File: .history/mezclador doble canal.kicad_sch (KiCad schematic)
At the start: 40 parts, among them J1 Conn_Coaxial, J3 Conn_Coaxial, J4 Conn_Coaxial, J5 Conn_Coaxial, J7 Screw_Terminal_01x02, J8 Conn_Coaxial, SW1 SW_SPST, U1 NE5532, U2 TL071

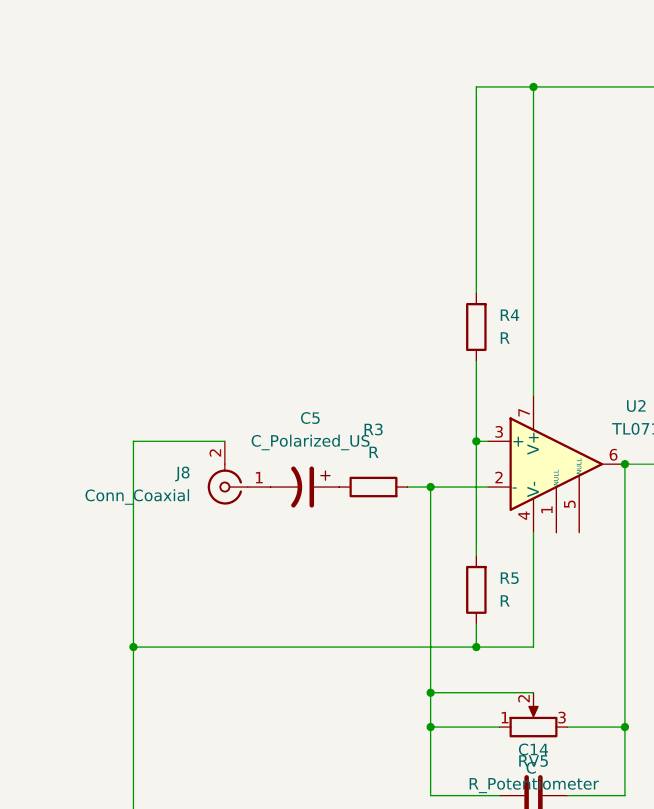
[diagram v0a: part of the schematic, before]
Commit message: acomodando componentes
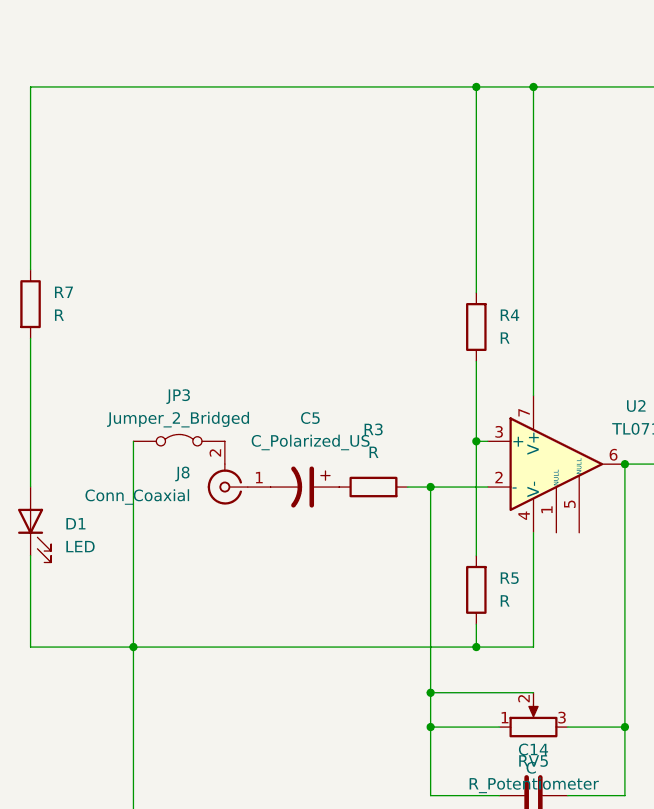
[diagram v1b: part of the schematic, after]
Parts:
- added D1: LED, LED_THT:LED_D5.0mm, symbol Device:LED
- added JP3: Jumper_2_Bridged, personal:Jumper_Wire_7mm, symbol Jumper:Jumper_2_Bridged
- added R7: R, Resistor_THT:R_Axial_DIN0207_L6.3mm_D2.5mm_P7.62mm_Horizontal, symbol Device:R
- JP2: footprint personal:Jumper_Wire_10mm -> personal:Jumper_Wire_7mm
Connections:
- net GND: now also D1.1 (K), JP3.1 (A); no longer J8.2 (Ext)
- net VCC: now also R7.1
- new net: J8.2 (Ext), JP3.2 (B)
- new net: D1.2 (A), R7.2

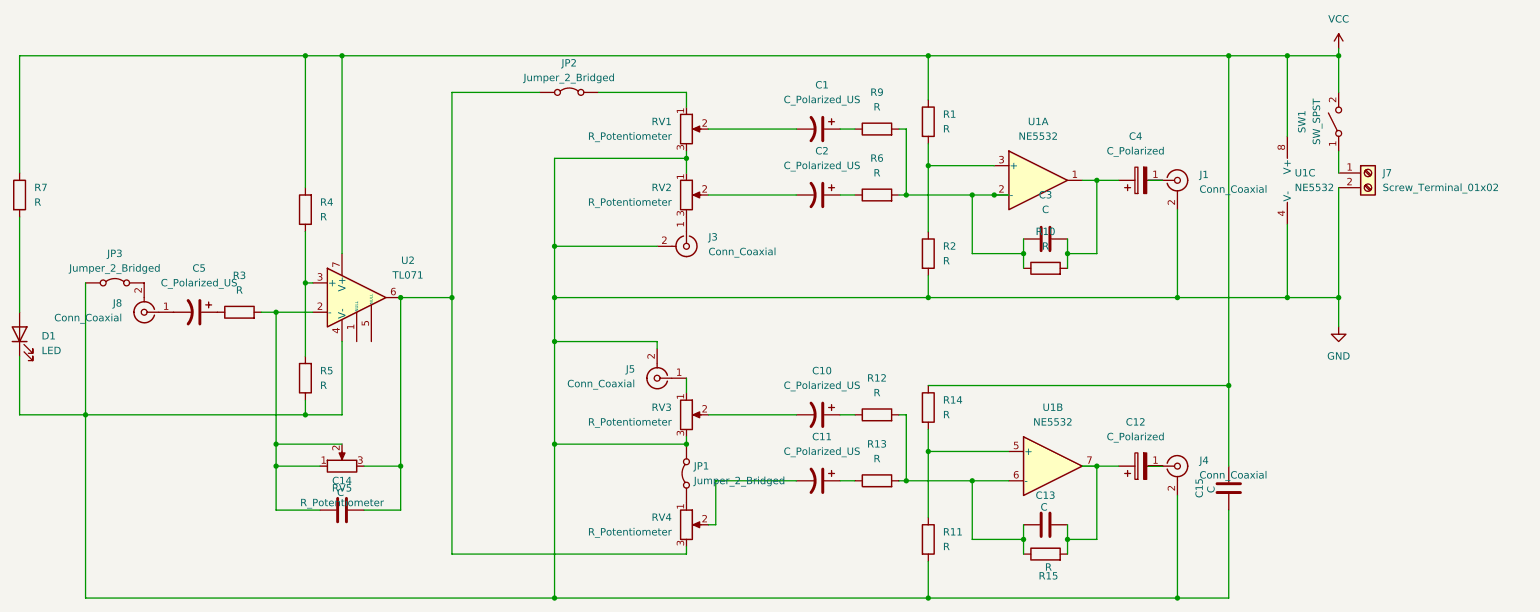
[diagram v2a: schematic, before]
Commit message: todo en su lugar / tamaño 50x55
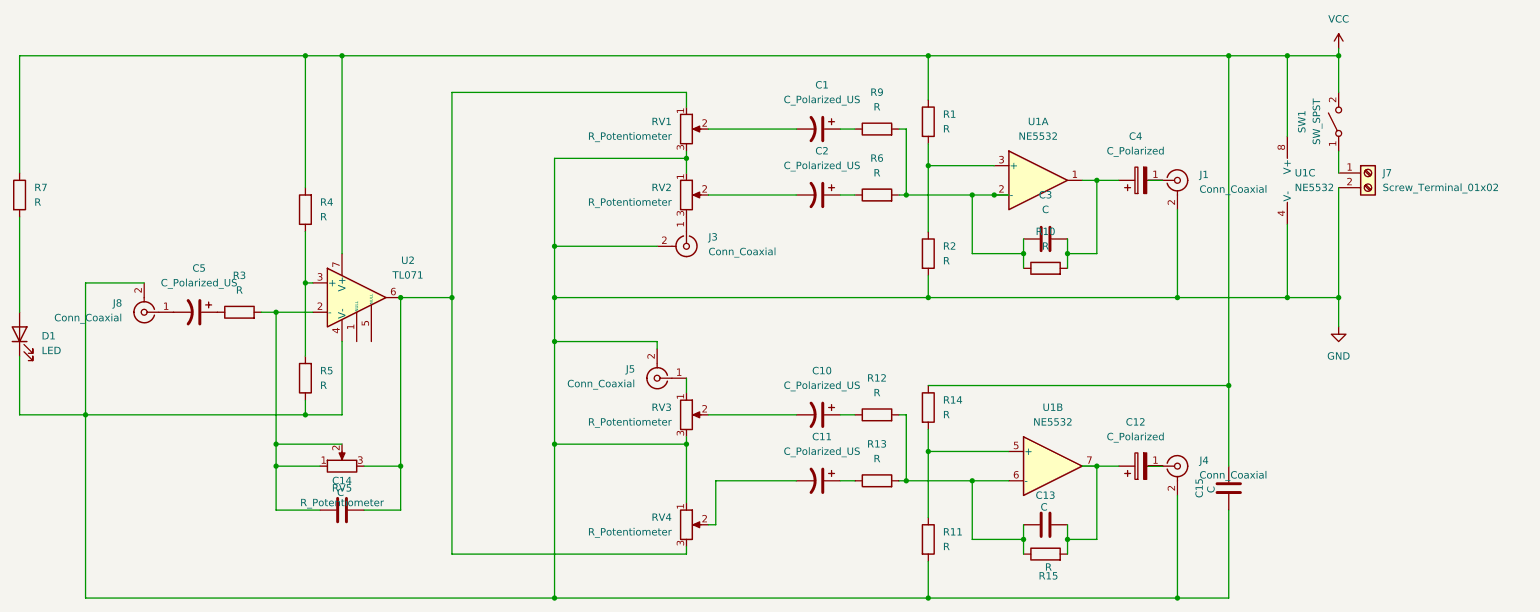
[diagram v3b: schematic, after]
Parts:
- removed JP1: Jumper_2_Bridged, personal:Jumper_Wire_10mm, symbol Jumper:Jumper_2_Bridged
- removed JP2, JP3: Jumper_2_Bridged, personal:Jumper_Wire_7mm, symbol Jumper:Jumper_2_Bridged
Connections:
- net GND: now also J8.2 (Ext), RV4.1
- net at C14.2, RV4.3, RV5.3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: now also RV1.1
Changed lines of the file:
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@@
 	(paper "A4")
 	(junction
+		(at 142.24 95.25)
+		(diameter 0)
+		(color 0 0 0 0)
+	)
+	(junction
 		(at 208.28 62.23)
 		(diameter 0)
@@
 	)
 	(junction
-		(at 142.24 95.25)
-		(diameter 0)
-		(color 0 0 0 0)
-	)
-	(junction
 		(at 184.15 69.85)
 		(diameter 0)
@@
 	(wire
 		(pts
-			(xy 127 34.29) (xy 142.24 34.29)
-		)
-		(stroke
-			(width 0)
-			(type default)
-		)
-	)
-	(wire
-		(pts
 			(xy 208.28 62.23) (xy 208.28 64.77)
 		)
@@
 	(wire
 		(pts
+			(xy 38.1 67.31) (xy 48.26 67.31)
+		)
+		(stroke
+			(width 0)
+			(type default)
+		)
+	)
+	(wire
+		(pts
 			(xy 119.38 69.85) (xy 119.38 77.47)
 		)
@@
 	(wire
 		(pts
+			(xy 142.24 95.25) (xy 142.24 105.41)
+		)
+		(stroke
+			(width 0)
+			(type default)
+		)
+	)
+	(wire
+		(pts
 			(xy 26.67 80.01) (xy 26.67 90.17)
 		)
@@
 	(wire
 		(pts
-			(xy 101.6 34.29) (xy 116.84 34.29)
+			(xy 101.6 34.29) (xy 142.24 34.29)
 		)
 		(stroke
@@
 	)
 	(symbol
-		(lib_id "Jumper:Jumper_2_Bridged")
-		(at 142.24 100.33 90)
-		(unit 1)
-		(body_style 1)
-		(exclude_from_sim no)
-		(in_bom yes)
-		(on_board yes)
-		(in_pos_files yes)
-		(dnp no)
-		(fields_autoplaced yes)
-		(property "Reference" "JP1"
-			(at 143.51 99.0599 90)
-			(show_name no)
-			(do_not_autoplace no)
-			(effects
-				(font
-					(size 1.27 1.27)
-				)
-				(justify right)
-			)
-		)
-		(property "Value" "Jumper_2_Bridged"
-			(at 143.51 101.5999 90)
-			(show_name no)
-			(do_not_autoplace no)
-			(effects
-				(font
-					(size 1.27 1.27)
-				)
-				(justify right)
-			)
-		)
-		(property "Footprint" "personal:Jumper_Wire_10mm"
-			(at 142.24 100.33 0)
-			(hide yes)
-			(show_name no)
-			(do_not_autoplace no)
-			(effects
-				(font
-					(size 1.27 1.27)
-				)
-			)
-		)
-		(property "Datasheet" ""
-			(at 147.32 100.33 0)
-			(hide yes)
-			(show_name no)
-			(do_not_autoplace no)
-			(effects
-				(font
-					(size 1.27 1.27)
-				)
-			)
-		)
-		(property "Description" "Jumper, 2-pole, closed/bridged"
-			(at 149.86 100.33 0)
-			(hide yes)
-			(show_name no)
-			(do_not_autoplace no)
-			(effects
-				(font
-					(size 1.27 1.27)
-				)
-			)
-		)
-		(pin "2"
-		)
-		(pin "1"
-		)
-		(instances
-			(project "mezclador doble canal"
-				(path "/1fd6db7d-bb33-43be-9c70-fde303eb7f84"
-					(reference "JP1")
-					(unit 1)
-				)
-			)
-		)
-	)
-	(symbol
 		(lib_id "Device:C")
 		(at 204.47 109.22 90)
@@
 	)
 	(symbol
-		(lib_id "Jumper:Jumper_2_Bridged")
-		(at 121.92 34.29 0)
-		(unit 1)
-		(body_style 1)
-		(exclude_from_sim no)
-		(in_bom yes)
-		(on_board yes)
-		(in_pos_files yes)
-		(dnp no)
-		(fields_autoplaced yes)
-		(property "Reference" "JP2"
-			(at 121.92 29.21 0)
-			(show_name no)
-			(do_not_autoplace no)
-			(effects
-				(font
-					(size 1.27 1.27)
-				)
-			)
-		)
-		(property "Value" "Jumper_2_Bridged"
-			(at 121.92 31.75 0)
-			(show_name no)
-			(do_not_autoplace no)
-			(effects
-				(font
-					(size 1.27 1.27)
-				)
-			)
-		)
-		(property "Footprint" "personal:Jumper_Wire_7mm"
-			(at 121.92 34.29 0)
-			(hide yes)
-			(show_name no)
-			(do_not_autoplace no)
-			(effects
-				(font
-					(size 1.27 1.27)
-				)
-			)
-		)
-		(property "Datasheet" ""
-			(at 121.92 39.37 0)
-			(hide yes)
-			(show_name no)
-			(do_not_autoplace no)
-			(effects
-				(font
-					(size 1.27 1.27)
-				)
-			)
-		)
-		(property "Description" "Jumper, 2-pole, closed/bridged"
-			(at 121.92 41.91 0)
-			(hide yes)
-			(show_name no)
-			(do_not_autoplace no)
-			(effects
-				(font
-					(size 1.27 1.27)
-				)
-			)
-		)
-		(pin "1"
-		)
-		(pin "2"
-		)
-		(instances
-			(project "mezclador doble canal"
-				(path "/1fd6db7d-bb33-43be-9c70-fde303eb7f84"
-					(reference "JP2")
-					(unit 1)
-				)
-			)
-		)
-	)
-	(symbol
 		(lib_id "Device:R")
 		(at 76.2 54.61 180)
@@
 					(unit 1)
 				)
-			)
-		)
-	)
-	(symbol
-		(lib_id "Jumper:Jumper_2_Bridged")
-		(at 43.18 67.31 0)
-		(unit 1)
-		(body_style 1)
-		(exclude_from_sim no)
-		(in_bom yes)
-		(on_board yes)
-		(in_pos_files yes)
-		(dnp no)
-		(fields_autoplaced yes)
-		(property "Reference" "JP3"
-			(at 43.18 62.23 0)
-			(show_name no)
-			(do_not_autoplace no)
-			(effects
-				(font
-					(size 1.27 1.27)
-				)
-			)
-		)
-		(property "Value" "Jumper_2_Bridged"
-			(at 43.18 64.77 0)
-			(show_name no)
-			(do_not_autoplace no)
-			(effects
-				(font
-					(size 1.27 1.27)
-				)
-			)
-		)
-		(property "Footprint" "personal:Jumper_Wire_7mm"
-			(at 43.18 67.31 0)
-			(hide yes)
-			(show_name no)
-			(do_not_autoplace no)
-			(effects
-				(font
-					(size 1.27 1.27)
-				)
-			)
-		)
-		(property "Datasheet" ""
-			(at 43.18 72.39 0)
-			(hide yes)
-			(show_name no)
-			(do_not_autoplace no)
-			(effects
-				(font
-					(size 1.27 1.27)
-				)
-			)
-		)
-		(property "Description" "Jumper, 2-pole, closed/bridged"
-			(at 43.18 74.93 0)
-			(hide yes)
-			(show_name no)
-			(do_not_autoplace no)
-			(effects
-				(font
-					(size 1.27 1.27)
-				)
-			)
-		)
-		(pin "2"
-		)
-		(pin "1"
-		)
-		(instances
-			(project "mezclador doble canal"
-				(path "/1fd6db7d-bb33-43be-9c70-fde303eb7f84"
-					(reference "JP3")
-					(unit 1)
-				)

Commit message: todo acomodado - corregir etiquetas
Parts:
- D1: footprint LED_THT:LED_D5.0mm -> personal:double wire
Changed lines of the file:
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@@
 			)
 		)
-		(property "Footprint" "LED_THT:LED_D5.0mm"
+		(property "Footprint" "personal:double wire"
 			(at 26.67 76.2 0)
 			(hide yes)

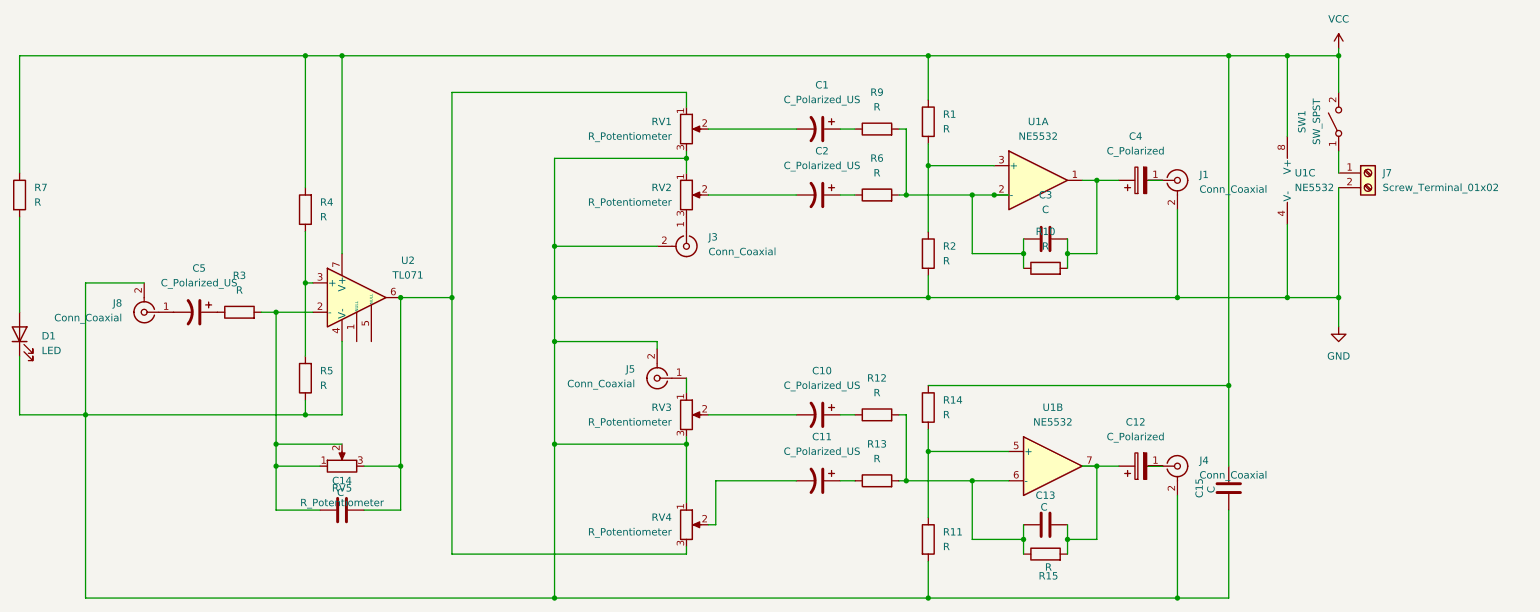
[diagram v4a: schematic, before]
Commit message: depurando proyecto
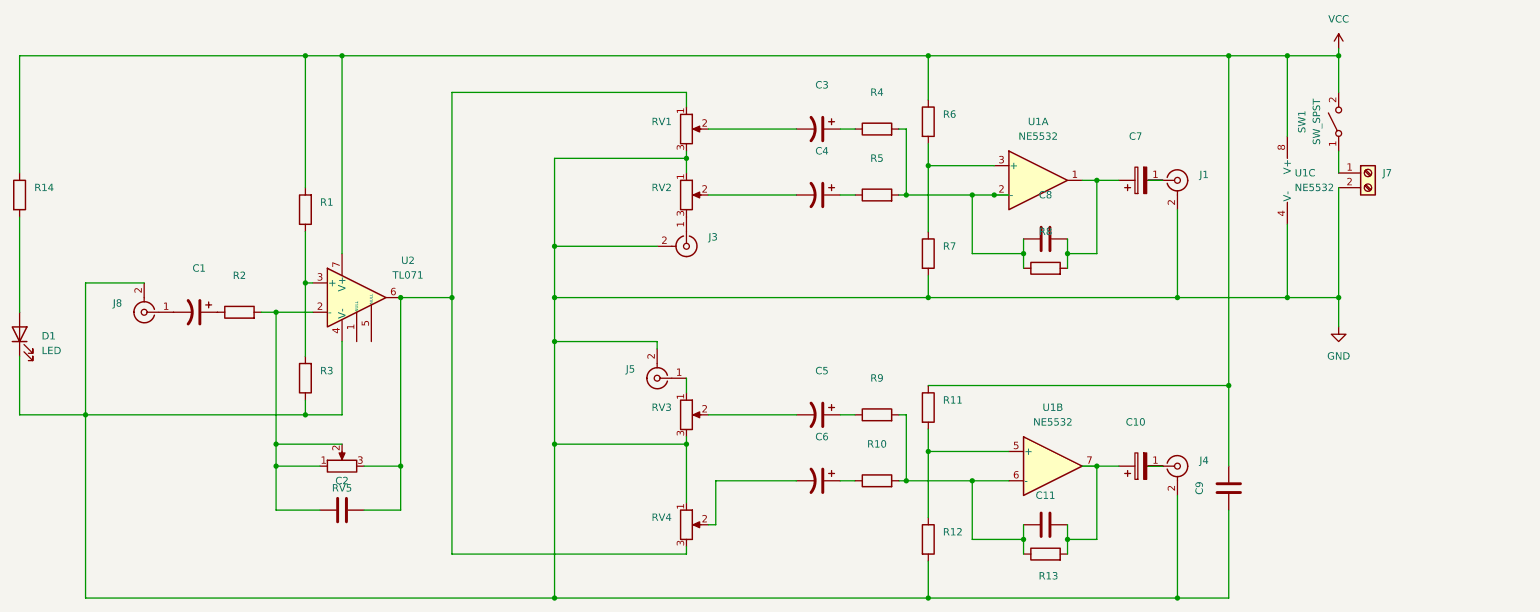
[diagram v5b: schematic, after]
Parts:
- renumbered C5 to C1, C12 to C10, C13 to C11, C14 to C2, C1 to C3, C2 to C4, C10 to C5, C11 to C6, C4 to C7, C3 to C8, C15 to C9, R4 to R1, R13 to R10, R14 to R11, R11 to R12, R15 to R13, R7 to R14, R3 to R2, R5 to R3, R9 to R4, R6 to R5, R1 to R6, R2 to R7, R10 to R8, R12 to R9
